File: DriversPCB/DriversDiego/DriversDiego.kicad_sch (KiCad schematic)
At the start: 35 parts, among them IC1 DRV8411PWPR, IC2 DRV8411PWPR, IC3 DRV8411PWPR, J1 TB0012-508-02GR, J10 TB0012-508-02GR, J11 TB0012-508-02GR, J12 TB0012-508-02GR, J13 TB0012-508-02GR, J14 TB0012-508-02GR, J15 TB0012-508-02GR, J16 TB0012-508-02GR, J17 TB0012-508-02GR, J18 TB0012-508-02GR, J19 TB0012-508-02GR, J2 TB0012-508-02GR, J3 TB0012-508-02GR, J4 TB0012-508-02GR, J5 TB0012-508-02GR, J6 TB0012-508-02GR, J7 TB0012-508-02GR, J8 TB0012-508-02GR, J9 TB0012-508-02GR, U1 DRV8871DDA

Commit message: Zona cobre...
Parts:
- C1: footprint WCAP-CSGP_0805_H1.25:WCAP-CSGP_0805_H1.25_R -> Kicad_TitoSync_Footprints:WCAP-CSGP_0805_H1.25_R
- C3: footprint CL21B106KOQNFNE:CAPC2012X140N -> Kicad_TitoSync_Footprints:CAPC2012X140N
- IC1, IC2, IC3: footprint DRV8411PWPR:PWP0016C-IPC_A -> Kicad_TitoSync_Footprints:PWP0016C-IPC_A
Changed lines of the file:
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@@
 			)
 		)
-		(property "Footprint" "DRV8411PWPR:PWP0016C-IPC_A"
+		(property "Footprint" "Kicad_TitoSync_Footprints:PWP0016C-IPC_A"
 			(at 226.06 58.42 0)
 			(effects
@@
 			)
 		)
-		(property "Footprint" "DRV8411PWPR:PWP0016C-IPC_A"
+		(property "Footprint" "Kicad_TitoSync_Footprints:PWP0016C-IPC_A"
 			(at 95.25 109.22 0)
 			(effects
@@
 			)
 		)
-		(property "Footprint" "CL21B106KOQNFNE:CAPC2012X140N"
+		(property "Footprint" "Kicad_TitoSync_Footprints:CAPC2012X140N"
 			(at 196.85 31.75 0)
 			(effects
@@
 			)
 		)
-		(property "Footprint" "DRV8411PWPR:PWP0016C-IPC_A"
+		(property "Footprint" "Kicad_TitoSync_Footprints:PWP0016C-IPC_A"
 			(at 219.71 139.7 0)
 			(effects
@@
 			)
 		)
-		(property "Footprint" "WCAP-CSGP_0805_H1.25:WCAP-CSGP_0805_H1.25_R"
+		(property "Footprint" "Kicad_TitoSync_Footprints:WCAP-CSGP_0805_H1.25_R"
 			(at 114.3 38.1 0)
 			(effects

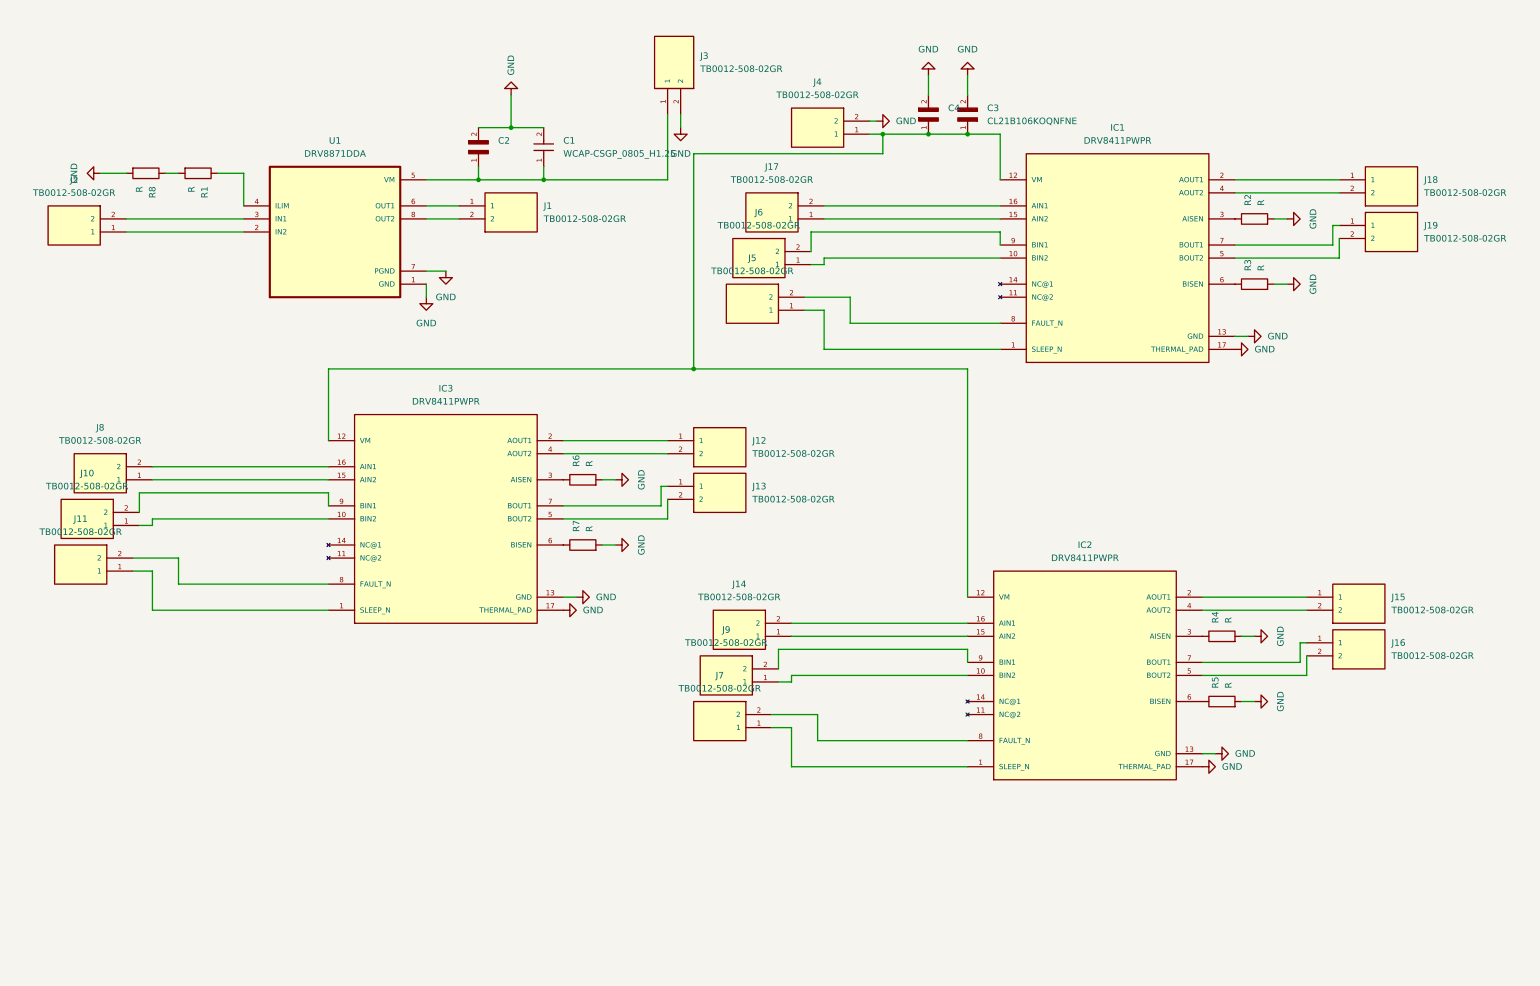
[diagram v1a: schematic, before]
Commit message: Last PCB revision
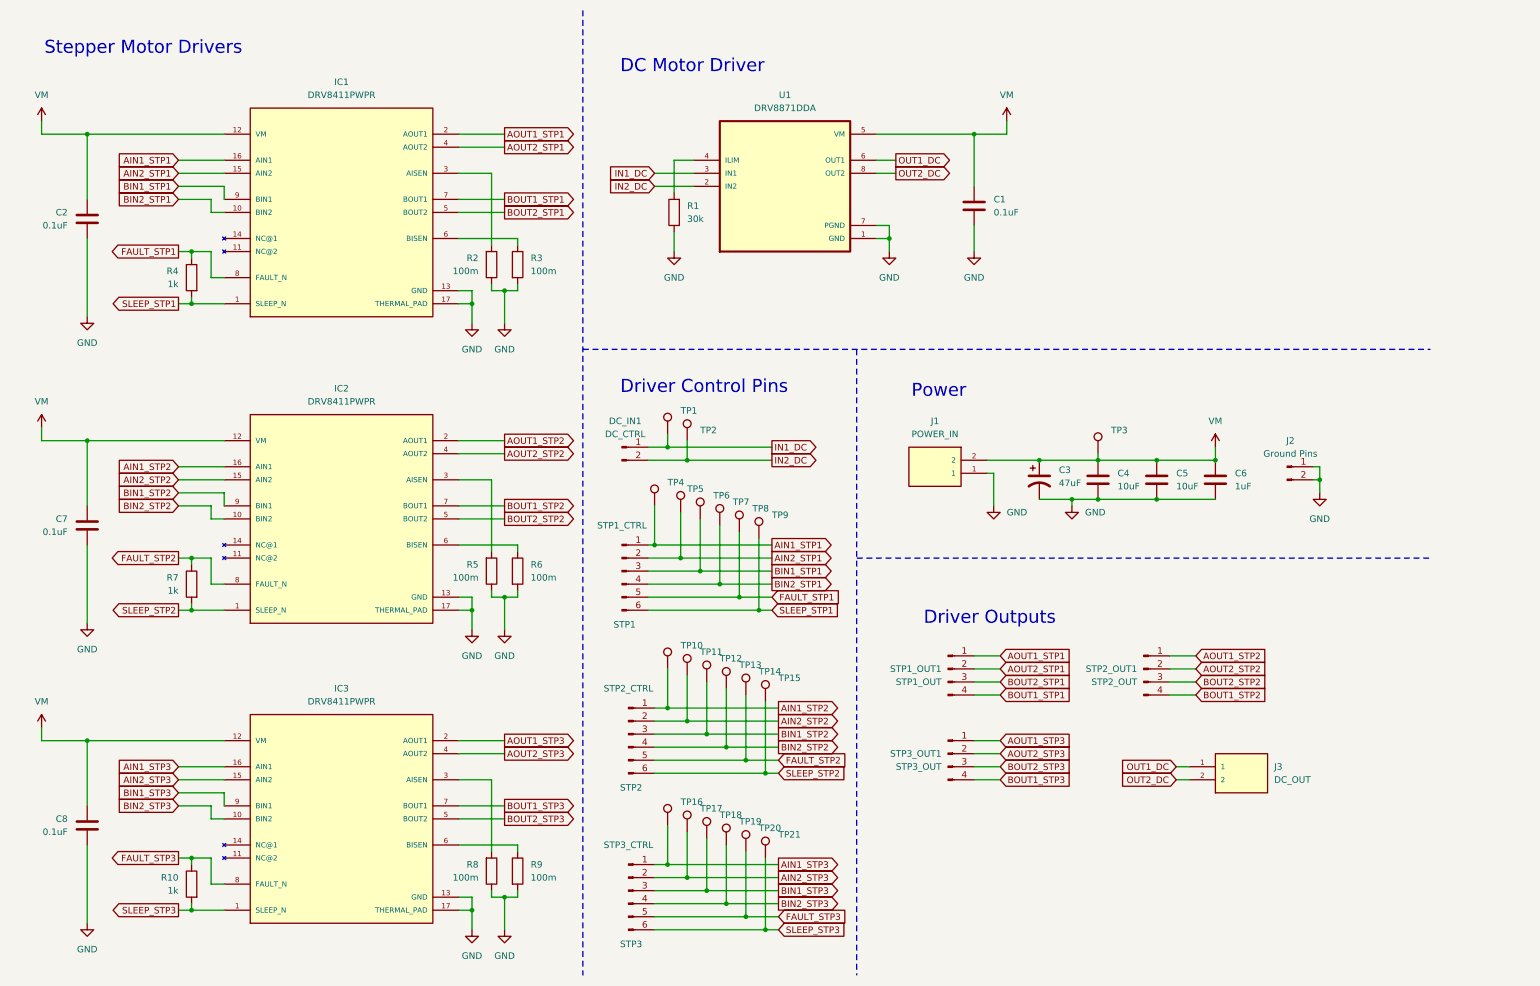
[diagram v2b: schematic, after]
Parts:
- removed C1: WCAP-CSGP_0805_H1.25, Kicad_TitoSync_Footprints:WCAP-CSGP_0805_H1.25_R, symbol WCAP-CSGP_0805_H1.25:WCAP-CSGP_0805_H1.25
- removed C3: CL21B106KOQNFNE, Kicad_TitoSync_Footprints:CAPC2012X140N, symbol CL21B106KOQNFNE:CL21B106KOQNFNE
- removed IC2: DRV8411PWPR, Kicad_TitoSync_Footprints:PWP0016C-IPC_A, symbol DRV8411PWPR:DRV8411PWPR
- removed J1, J10, J11, J12, J13, J14, J15, J16, J17, J18, J19, J2, J5, J6, J7, J8, J9: TB0012-508-02GR, Kicad_TitoSync_Footprints:SAMESKY_TB0012-508-02GR, symbol TB0012-508-02GR:TB0012-508-02GR
- added C2, C8: 0.1uF, Capacitor_SMD:C_0402_1005Metric, symbol Device:C
- added C3: 47uF, Capacitor_SMD:CP_Elec_6.3x5.4, symbol Device:C_Polarized_US
- added C4, C5: 10uF, Capacitor_SMD:C_1206_3216Metric, symbol Device:C
- added C6: 1uF, Capacitor_SMD:C_0603_1608Metric, symbol Device:C
- added DC_IN1: DC_CTRL, Connector_PinHeader_2.54mm:PinHeader_1x02_P2.54mm_Vertical, symbol Connector:Conn_01x02_Pin
- added IC1: DRV8411PWPR, Package_SO:HTSSOP-16-1EP_4.4x5mm_P0.65mm_EP3.4x5mm_Mask2.66x2.46mm, symbol DRV8411PWPR:DRV8411PWPR
- added J2: Ground Pins, Connector_PinHeader_2.54mm:PinHeader_1x02_P2.54mm_Vertical, symbol Connector:Conn_01x02_Pin
- added R10: 1k, Resistor_SMD:R_0805_2012Metric_Pad1.20x1.40mm_HandSolder, symbol Device:R
- added R9: 100m, Resistor_SMD:R_1206_3216Metric, symbol Device:R
- added STP1: STP1_CTRL, Connector_PinHeader_2.54mm:PinHeader_1x06_P2.54mm_Vertical, symbol Connector:Conn_01x06_Pin
- added STP1_OUT1: STP1_OUT, Connector_PinHeader_2.54mm:PinHeader_1x04_P2.54mm_Vertical, symbol Connector:Conn_01x04_Pin
- added STP2: STP2_CTRL, Connector_PinHeader_2.54mm:PinHeader_1x06_P2.54mm_Vertical, symbol Connector:Conn_01x06_Pin
- added STP2_OUT1: STP2_OUT, Connector_PinHeader_2.54mm:PinHeader_1x04_P2.54mm_Vertical, symbol Connector:Conn_01x04_Pin
- added STP3: STP3_CTRL, Connector_PinHeader_2.54mm:PinHeader_1x06_P2.54mm_Vertical, symbol Connector:Conn_01x06_Pin
- added STP3_OUT1: STP3_OUT, Connector_PinHeader_2.54mm:PinHeader_1x04_P2.54mm_Vertical, symbol Connector:Conn_01x04_Pin
- added TP1, TP10, TP11, TP12, TP13, TP14, TP15, TP16, TP17, TP18, TP19, TP2, TP20, TP21, TP3, TP4, TP5, TP6, TP7, TP8, TP9: TestPoint, TestPoint:TestPoint_Keystone_5019_Miniature, symbol Connector:TestPoint
- C1: renamed from C2; value 500R15Y104MV4T -> 0.1uF; footprint Kicad_TitoSync_Footprints:CAPC2012X127N -> Capacitor_SMD:C_0402_1005Metric; symbol 500R15Y104MV4T:500R15Y104MV4T -> Device:C; A_MAX 1.27 -> (none); A_MIN 1.27 -> (none); A_NOM 1.27 -> (none); Check_prices https://www.snapeda.com/parts/500R15Y104MV4T/Johanson/view-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 -> (none); D_MAX 2.28 -> (none); D_MIN 1.78 -> (none); D_NOM 2.03 -> (none); Description_1 Mlcc 0805, 0.1 f, 20%, 50v -> (none); E_MAX 1.52 -> (none); E_MIN 1.02 -> (none); E_NOM 1.27 -> (none); L1_MAX 0.76 -> (none); L1_MIN 0.26 -> (none); L1_NOM 0.51 -> (none); L_MAX 0.76 -> (none); L_MIN 0.26 -> (none); L_NOM 0.51 -> (none); MF Johanson -> (none); MP 500R15Y104MV4T -> (none); Manufacturer (none) -> MuRata; PartNumber (none) -> GRM155R71H104KE14D; Price None -> (none); STANDARD IPC-7351B -> (none); SnapEDA_Link https://www.snapeda.com/parts/500R15Y104MV4T/Johanson/view-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 -> (none)
- C7: renamed from C4; value 500R15Y104MV4T -> 0.1uF; footprint Kicad_TitoSync_Footprints:EXV-9B_KEM -> Capacitor_SMD:C_0402_1005Metric; symbol 500R15Y104MV4T:500R15Y104MV4T -> Device:C; A_MAX 1.27 -> (none); A_MIN 1.27 -> (none); A_NOM 1.27 -> (none); Check_prices https://www.snapeda.com/parts/500R15Y104MV4T/Johanson/view-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 -> (none); D_MAX 2.28 -> (none); D_MIN 1.78 -> (none); D_NOM 2.03 -> (none); Description_1 Mlcc 0805, 0.1 f, 20%, 50v -> (none); E_MAX 1.52 -> (none); E_MIN 1.02 -> (none); E_NOM 1.27 -> (none); L1_MAX 0.76 -> (none); L1_MIN 0.26 -> (none); L1_NOM 0.51 -> (none); L_MAX 0.76 -> (none); L_MIN 0.26 -> (none); L_NOM 0.51 -> (none); MF Johanson -> (none); MP 500R15Y104MV4T -> (none); Manufacturer (none) -> MuRata; PartNumber (none) -> GRM155R71H104KE14D; Price None -> (none); STANDARD IPC-7351B -> (none); SnapEDA_Link https://www.snapeda.com/parts/500R15Y104MV4T/Johanson/view-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 -> (none)
- IC2: renamed from IC1; footprint Kicad_TitoSync_Footprints:PWP0016C-IPC_A -> Package_SO:HTSSOP-16-1EP_4.4x5mm_P0.65mm_EP3.4x5mm_Mask2.66x2.46mm; Check_prices https://www.snapeda.com/parts/DRV8411PWPR/Texas+Instruments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 -> (none); Description_1 1.65-V to 11-V, 4-A, dual H-bridge motor driver with curren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 -> (none); MF Texas Instruments -> (none); MP DRV8411PWPR -> (none); Manufacturer (none) -> Texas Instruments; PartNumber (none) -> DRV8411PWPR; Price None -> (none); SnapEDA_Link https://www.snapeda.com/parts/DRV8411PWPR/Texas+Instruments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 -> (none)
- IC3: footprint Kicad_TitoSync_Footprints:PWP0016C-IPC_A -> Package_SO:HTSSOP-16-1EP_4.4x5mm_P0.65mm_EP3.4x5mm_Mask2.66x2.46mm; Check_prices https://www.snapeda.com/parts/DRV8411PWPR/Texas+Instruments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 -> (none); Description_1 1.65-V to 11-V, 4-A, dual H-bridge motor driver with curren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 -> (none); MF Texas Instruments -> (none); MP DRV8411PWPR -> (none); Manufacturer (none) -> Texas Instruments; PartNumber (none) -> DRV8411PWPR; Price None -> (none); SnapEDA_Link https://www.snapeda.com/parts/DRV8411PWPR/Texas+Instruments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 -> (none)
- J1: renamed from J4; value TB0012-508-02GR -> POWER_IN; footprint Kicad_TitoSync_Footprints:SAMESKY_TB0012-508-02GR -> TerminalBlock_MetzConnect:TerminalBlock_MetzConnect_Type094_RT03502HBLU_1x02_P5.00mm_Horizontal; CREATOR ASHISH -> (none); Check_prices https://www.snapeda.com/parts/TB0012-508-02GR/Same+Sky/view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 -> (none); Description_1 2 Position Wire to Board Terminal Block Horizontal with Boa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 -> (none); MANUFACTURER Same Sky -> (none); MAXIMUM_PACKAGE_HEIGHT 19.2mm -> (none); MF Same Sky (Formerly CUI Devices) -> (none); MP TB0012-508-02GR -> (none); Manufacturer (none) -> Same Sky (Formerly CUI Devices); PartNumber (none) -> TB0012-508-02GR; Price None -> (none); STANDARD Manufacturer Recommendations -> (none); SnapEDA_Link https://www.snapeda.com/parts/TB0012-508-02GR/Same+Sky/view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 -> (none)
- J3: value TB0012-508-02GR -> DC_OUT; footprint Kicad_TitoSync_Footprints:SAMESKY_TB0012-508-02GR -> TerminalBlock_MetzConnect:TerminalBlock_MetzConnect_Type094_RT03502HBLU_1x02_P5.00mm_Horizontal; CREATOR ASHISH -> (none); Check_prices https://www.snapeda.com/parts/TB0012-508-02GR/Same+Sky/view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 -> (none); Description_1 2 Position Wire to Board Terminal Block Horizontal with Boa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 -> (none); MANUFACTURER Same Sky -> (none); MAXIMUM_PACKAGE_HEIGHT 19.2mm -> (none); MF Same Sky (Formerly CUI Devices) -> (none); MP TB0012-508-02GR -> (none); Manufacturer (none) -> Same Sky (Formerly CUI Devices); PartNumber (none) -> TB0012-508-02GR; Price None -> (none); STANDARD Manufacturer Recommendations -> (none); SnapEDA_Link https://www.snapeda.com/parts/TB0012-508-02GR/Same+Sky/view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 -> (none)
- R1: value R -> 30k; Manufacturer (none) -> Stackpole Electronics Inc
- R2, R3, R5, R6, R8: value R -> 100m; footprint Resistor_SMD:R_0805_2012Metric_Pad1.20x1.40mm_HandSolder -> Resistor_SMD:R_1206_3216Metric; Manufacturer (none) -> RESI; PartNumber (none) -> MFCR1206FR100QHR
- R4, R7: value R -> 1k; Manufacturer (none) -> Stackpole Electronics Inc
- U1: Check_prices https://www.snapeda.com/parts/DRV8871DDA/Texas+Instruments/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 -> (none); Description_1 50-V, 3.6-A H-bridge motor driver with integrated current s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 -> (none); MF Texas Instruments -> (none); MP DRV8871DDA -> (none); Manufacturer (none) -> Texas Instruments; PartNumber (none) -> DRV8871DDA; Price None -> (none); SnapEDA_Link https://www.snapeda.com/parts/DRV8871DDA/Texas+Instruments/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 -> (none)
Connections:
- net GND: now also C1.1, C7.1, J1.1, R1.1, R2.1, R5.1, R8.1, C2.1, C3.2, C4.1, C5.1, C6.2, C8.1, IC1.13 (GND), IC1.17 (THERMAL_PAD), J2.1 (Pin_1), J2.2 (Pin_2), R9.2; no longer C1.2, C7.2, J1.2, J3.2, R2.2, R4.2, R5.2, R7.2, R8.2
- net at R1.2: now also U1.4 (ILIM); no longer R8.1
- net BIN2_STP2: now reaches IC2.10 (BIN2)
- net BIN2_STP2: now also STP2.4 (Pin_4), TP13.1
- net BIN1_STP2: now reaches IC2.9 (BIN1)
- net BIN1_STP2: now also STP2.3 (Pin_3), TP12.1
- net IN2_DC: now reaches U1.2 (IN2)
- net IN2_DC: now also DC_IN1.2 (Pin_2), TP2.1
- net IN1_DC: now reaches U1.3 (IN1)
- net IN1_DC: now also DC_IN1.1 (Pin_1), TP1.1
- net AOUT1_STP2: now reaches IC2.2 (AOUT1)
- net AOUT1_STP2: now also STP2_OUT1.1 (Pin_1)
- net AOUT2_STP2: now reaches IC2.4 (AOUT2)
- net AOUT2_STP2: now also STP2_OUT1.2 (Pin_2)
- net AIN2_STP3: now reaches IC3.15 (AIN2)
- net AIN2_STP3: now also STP3.2 (Pin_2), TP17.1
- net AIN1_STP3: now reaches IC3.16 (AIN1)
- net AIN1_STP3: now also STP3.1 (Pin_1), TP16.1
- net FAULT_STP1: now reaches R4.1
- net FAULT_STP1: now also IC1.8 (FAULT_N), STP1.5 (Pin_5), TP8.1
- net SLEEP_STP2: now reaches IC2.1 (SLEEP_N)
- net SLEEP_STP2: now also R7.2, STP2.6 (Pin_6), TP15.1
- net VM: now reaches IC2.12 (VM), IC3.12 (VM)
- net VM: now also C1.2, C7.2, J1.2, U1.5 (VM), C2.2, C3.1, C4.2, C5.2, C6.1, C8.2, IC1.12 (VM), TP3.1; no longer C7.1, J1.1
- net AIN2_STP2: now reaches IC2.15 (AIN2)
- net AIN2_STP2: now also STP2.2 (Pin_2), TP11.1
- net AIN1_STP2: now reaches IC2.16 (AIN1)
- net AIN1_STP2: now also STP2.1 (Pin_1), TP10.1
- net at IC2.3 (AISEN): now also R5.2; no longer R2.1
- net BOUT2_STP2: now reaches IC2.5 (BOUT2)
- net BOUT2_STP2: now also STP2_OUT1.3 (Pin_3)
- net at IC2.6 (BISEN): now also R6.1; no longer R3.1
- net BOUT1_STP2: now reaches IC2.7 (BOUT1)
- net BOUT1_STP2: now also STP2_OUT1.4 (Pin_4)
- net FAULT_STP2: now reaches IC2.8 (FAULT_N)
- net FAULT_STP2: now also R7.1, STP2.5 (Pin_5), TP14.1
- net BIN2_STP3: now reaches IC3.10 (BIN2)
- net BIN2_STP3: now also STP3.4 (Pin_4), TP19.1
- net BIN1_STP3: now reaches IC3.9 (BIN1)
- net BIN1_STP3: now also STP3.3 (Pin_3), TP18.1
- net BOUT1_STP3: now reaches IC3.7 (BOUT1)
- net BOUT1_STP3: now also STP3_OUT1.4 (Pin_4)
- net BOUT2_STP3: now reaches IC3.5 (BOUT2)
- net BOUT2_STP3: now also STP3_OUT1.3 (Pin_3)
- net SLEEP_STP3: now reaches IC3.1 (SLEEP_N)
- net SLEEP_STP3: now also R10.2, STP3.6 (Pin_6), TP21.1
- net FAULT_STP3: now reaches IC3.8 (FAULT_N)
- net FAULT_STP3: now also R10.1, STP3.5 (Pin_5), TP20.1
- net AOUT1_STP3: now reaches IC3.2 (AOUT1)
- net AOUT1_STP3: now also STP3_OUT1.1 (Pin_1)
- net at IC3.3 (AISEN): now also R8.2; no longer R6.1
- net AOUT2_STP3: now reaches IC3.4 (AOUT2)
- net AOUT2_STP3: now also STP3_OUT1.2 (Pin_2)
- net at IC3.6 (BISEN): now also R9.1; no longer R7.1
- net OUT1_DC: now reaches U1.6 (OUT1)
- net OUT1_DC: now also J3.1
- net OUT2_DC: now reaches U1.8 (OUT2)
- net OUT2_DC: now also J3.2
- new net: IC1.3 (AISEN), R2.2
- new net: IC1.6 (BISEN), R3.1
- new net AIN1_STP1: IC1.16 (AIN1), STP1.1 (Pin_1), TP4.1
- new net AIN2_STP1: IC1.15 (AIN2), STP1.2 (Pin_2), TP5.1
- new net AOUT1_STP1: IC1.2 (AOUT1), STP1_OUT1.1 (Pin_1)
- new net AOUT2_STP1: IC1.4 (AOUT2), STP1_OUT1.2 (Pin_2)
- new net BIN1_STP1: IC1.9 (BIN1), STP1.3 (Pin_3), TP6.1
- new net BIN2_STP1: IC1.10 (BIN2), STP1.4 (Pin_4), TP7.1
- new net BOUT1_STP1: IC1.7 (BOUT1), STP1_OUT1.4 (Pin_4)
- new net BOUT2_STP1: IC1.5 (BOUT2), STP1_OUT1.3 (Pin_3)
- new net SLEEP_STP1: IC1.1 (SLEEP_N), R4.2, STP1.6 (Pin_6), TP9.1
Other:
- note added: "DC Motor Driver"
- note added: "Driver Control Pins"
- note added: "Driver Outputs"
- note added: "Power"
- note added: "Stepper Motor Drivers"
- moved on the sheet: IC2, J1, R1, U1
